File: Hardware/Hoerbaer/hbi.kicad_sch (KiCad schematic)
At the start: 49 parts, among them J6 PAW_A, J7 PAW_B, J8 PAW_C, J9 PAW_D, U2 PCF8574APWR, U3 PCF8574APWR, U4 PCF8574APWR, U5 TLC59108xPW, U6 TLC59108xPW, U7 TLC59108xPW

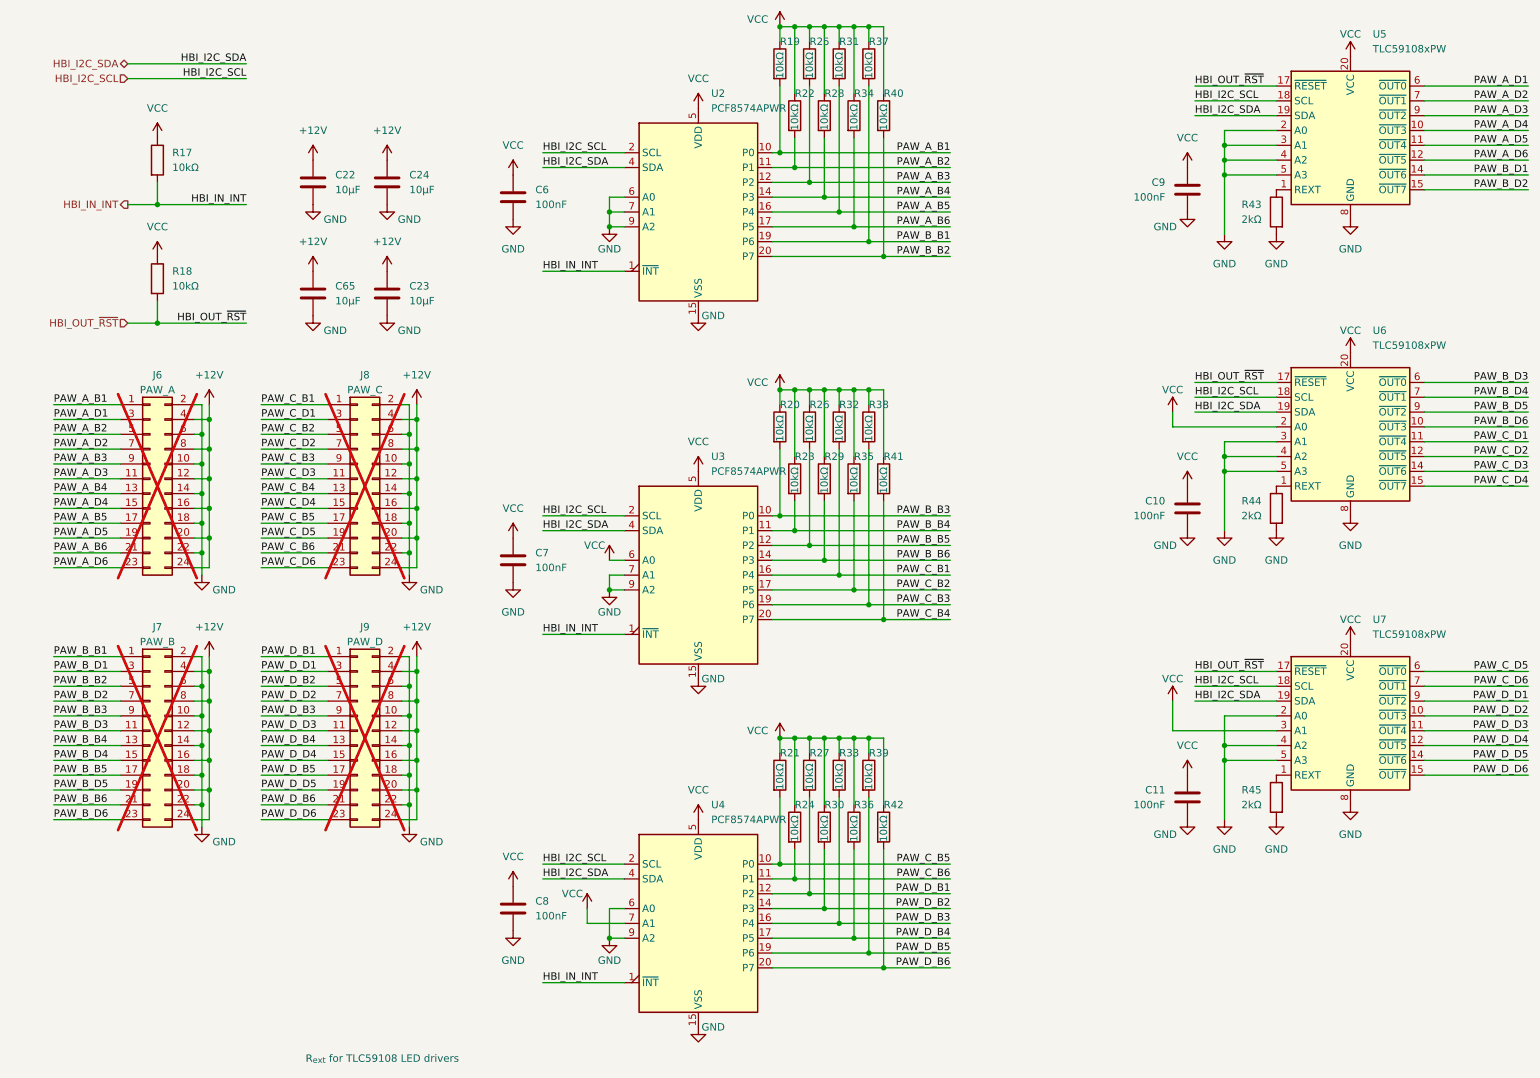
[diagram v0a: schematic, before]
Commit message: WIP new hw rev
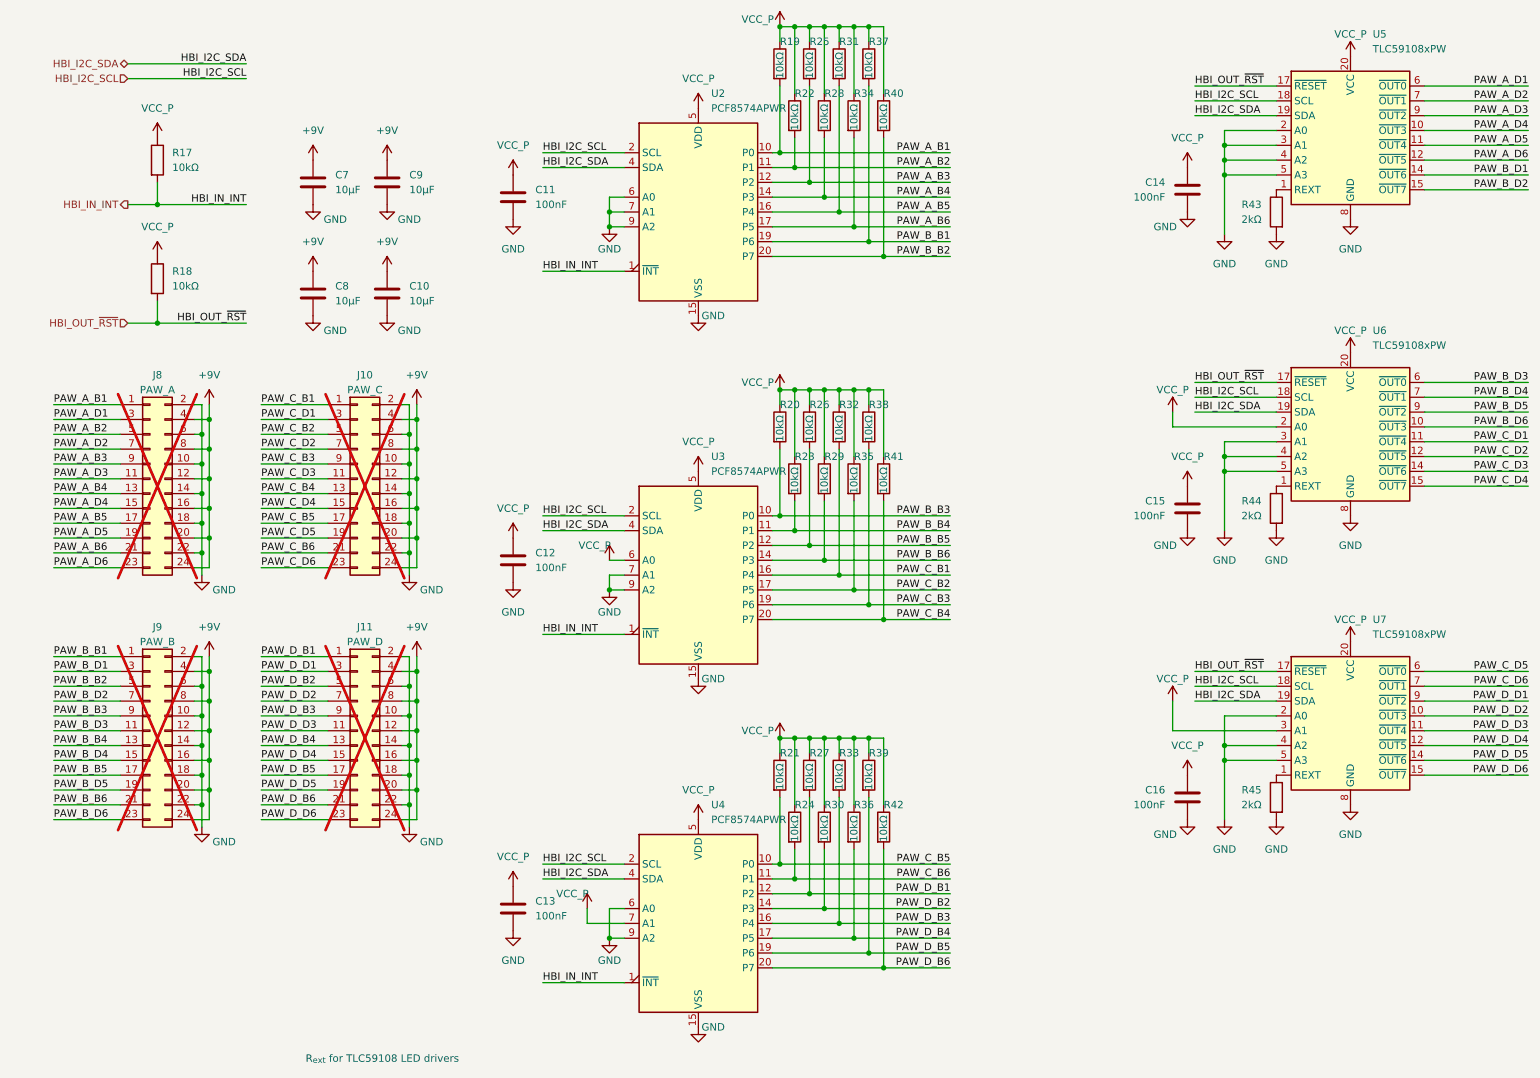
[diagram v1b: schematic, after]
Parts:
- renumbered C23 to C10, C6 to C11, C7 to C12, C8 to C13, C9 to C14, C10 to C15, C11 to C16, C22 to C7, C65 to C8, C24 to C9, J8 to J10, J9 to J11, J6 to J8, J7 to J9
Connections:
- net +12V renamed +9V
- net VCC renamed VCC_P
